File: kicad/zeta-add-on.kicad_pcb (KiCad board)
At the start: 2 copper layers, 29 x 35 mm, 14 parts

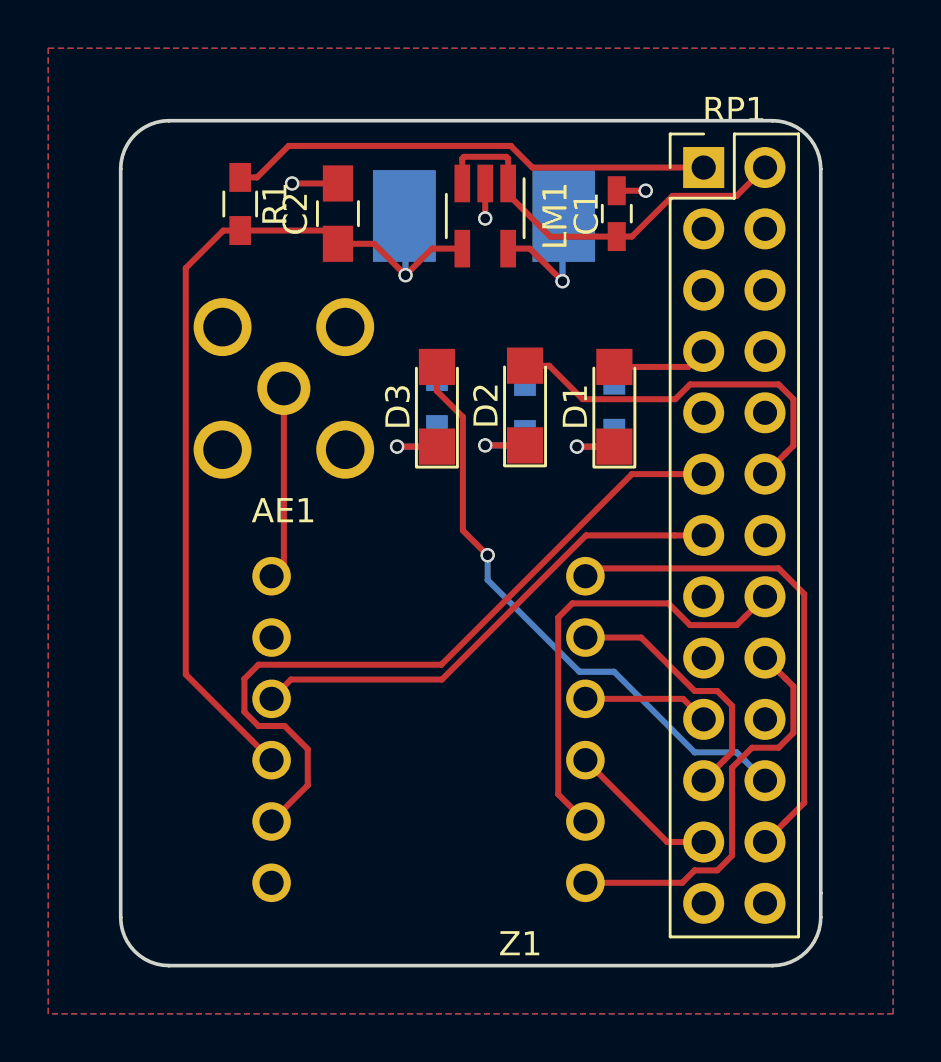
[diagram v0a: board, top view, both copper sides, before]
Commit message: finished board
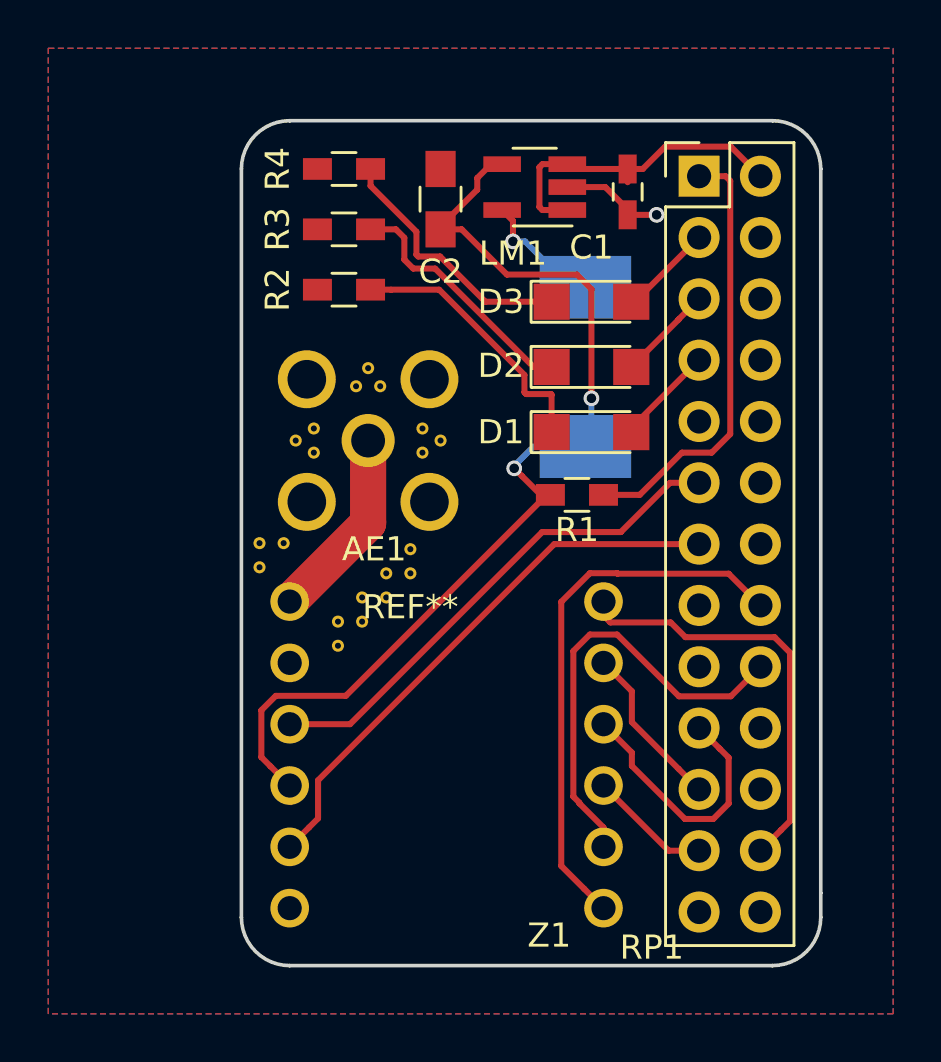
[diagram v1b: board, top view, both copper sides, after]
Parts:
- added REF**: STICH, STICH, F.Cu at (109.0, 116.8)
- added REF**: STICH, zeta-add-on:STICH, F.Cu at (107.8, 109.0)
- added REF**: STICH, zeta-add-on:STICH, F.Cu at (106.0, 110.8)
- added REF**: STICH, zeta-add-on:STICH, F.Cu at (106.0, 111.8)
- added REF**: STICH, zeta-add-on:STICH, F.Cu at (111.2, 111.2)
- added REF**: STICH, zeta-add-on:STICH, F.Cu at (108.2, 108.2)
- added REF**: STICH, zeta-add-on:STICH, F.Cu at (105.2, 111.2)
- added REF**: STICH, zeta-add-on:STICH, F.Cu at (110.0, 116.8)
- added REF**: STICH, zeta-add-on:STICH, F.Cu at (109.0, 117.8)
- added REF**: STICH, zeta-add-on:STICH, F.Cu at (108.0, 118.8)
- added REF**: STICH, zeta-add-on:STICH, F.Cu at (107.0, 119.8)
- added REF**: STICH, zeta-add-on:STICH, F.Cu at (110.0, 115.8)
- added REF**: STICH, zeta-add-on:STICH, F.Cu at (103.8, 115.5)
- added REF**: STICH, zeta-add-on:STICH, F.Cu at (108.0, 117.8)
- added REF**: STICH, zeta-add-on:STICH, F.Cu at (107.0, 118.8)
- added REF**: STICH, zeta-add-on:STICH, F.Cu at (104.8, 115.5)
- added REF**: STICH, zeta-add-on:STICH, F.Cu at (103.8, 116.5)
- added REF**: STICH, zeta-add-on:STICH, F.Cu at (110.5, 111.8)
- added REF**: STICH, zeta-add-on:STICH, F.Cu at (110.5, 110.8)
- added REF**: STICH, zeta-add-on:STICH, F.Cu at (108.8, 109.0)
- AE1: value Antenna -> Antenna_Shield
- R2, R3, R4: moved to F.Cu
- moved R1 18.4 mm to (116.9, 113.5), turned to 180 degrees
- moved R2 12.2 mm to (107.2, 105.0), turned to 0 degrees
- moved R3 10.5 mm to (107.2, 102.5), turned to 0 degrees
- moved R4 10.4 mm to (107.2, 100.0), turned to 0 degrees
- moved D3 7.74 mm to (117.5, 105.5), turned to 0 degrees
- moved L1 7.53 mm to (117.2, 108.2), turned to 90 degrees
- moved C2 4.29 mm to (111.2, 101.2)
- moved AE1 4.10 mm to (108.2, 111.2)
- moved D2 3.18 mm to (117.5, 108.2), turned to 0 degrees
- moved LM1 2.38 mm to (115.2, 100.8), turned to 180 degrees
- moved D1 1.42 mm to (117.5, 110.9), turned to 0 degrees
- moved Z1 1.29 mm to (111.5, 124.3)
- moved C1 1.01 mm to (119.0, 101.0), turned to 270 degrees
- moved RP1 0.41 mm to (122.0, 100.3)
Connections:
- RP1 pad 12: /LED2 -> (no net)
- RP1 pad 16: /GPIO1 -> /GPIO2
- RP1 pad 18: /GPIO2 -> /GPIO1
- RP1 pad 22: /LED3 -> (no net)
- RP1 pad 3: (no net) -> /LED3
- RP1 pad 5: (no net) -> /LED2
- Z1 pad 3: Net-(RP1-Pad13) -> Net-(RP1-Pad11)
- Z1 pad 5: Net-(RP1-Pad11) -> Net-(RP1-Pad13)
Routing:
- net /LED3: track 24.6 -> 3.91 mm, vias 1 -> 0
- net /LED2: track 15.8 -> 4.02 mm
- net Net-(RP1-Pad11): track 30.8 -> 21.1 mm
- net Net-(D1-Pad1): track 3.33 -> 11.3 mm, vias 1 -> 0
- net Net-(D2-Pad1): track 3.49 -> 11.1 mm, vias 1 -> 0
- net Net-(D3-Pad1): track 3.59 -> 10.7 mm, vias 1 -> 0
- net Net-(RP1-Pad19): track 5.25 -> 11.3 mm
- net /GPIO2: track 16.9 -> 22.7 mm
- net /3V3: track 37.6 -> 43.1 mm, vias 1 -> 2
- net Net-(RP1-Pad21): track 10.8 -> 6.88 mm
- net /5V: track 17.0 -> 13.3 mm
- net Net-(RP1-Pad24): track 20.6 -> 17.7 mm
- net Net-(RP1-Pad13): track 20.7 -> 23.1 mm
- net Net-(R1-Pad1): track 20.1 -> 18.2 mm
- net Net-(RP1-Pad23): track 6.30 -> 5.08 mm
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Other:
- board size 29 x 35 mm -> 24 x 35 mm
- net class Default: clearance 0.2 -> 0.25; via_dia 0.6 -> 0.65
- rule trace_clearance: 0.2 -> 0.25
- rule trace_min: 0.2 -> 0.1
- rule via_min_drill: 0.3 -> 0.2
- rule via_min_size: 0.4 -> 0.45
